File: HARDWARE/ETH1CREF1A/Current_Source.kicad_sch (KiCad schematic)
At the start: 25 parts, among them Q1102 BCP55, Q1103 BCP52, U1101 AD620, U1102 AD620

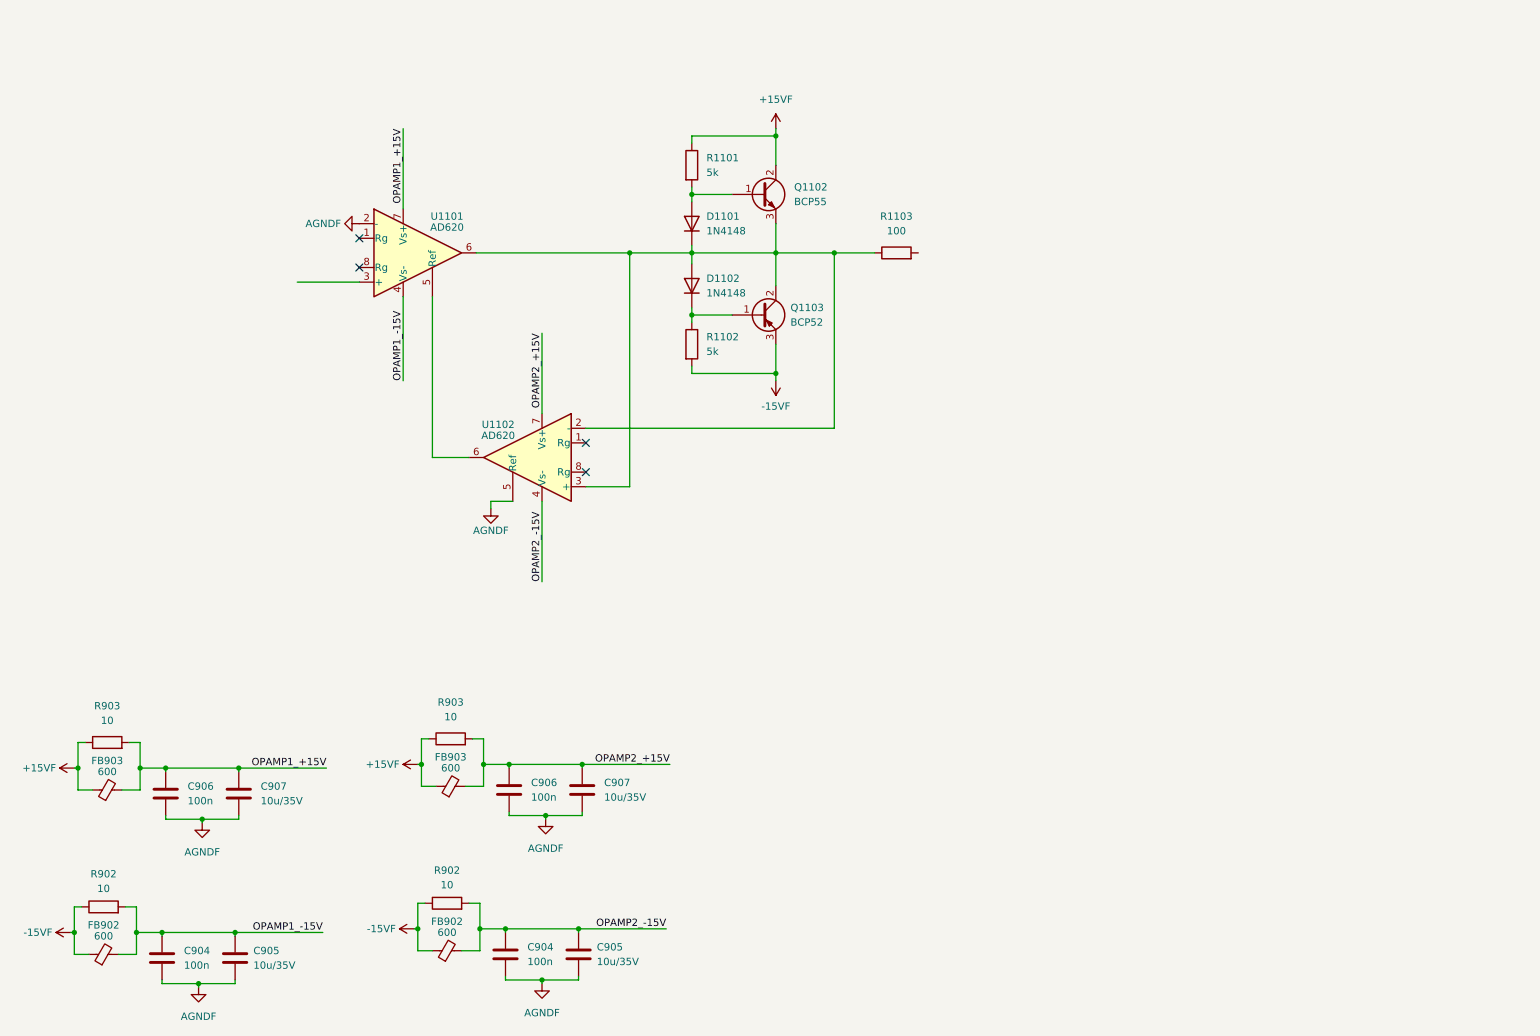
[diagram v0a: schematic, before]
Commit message: Hardware
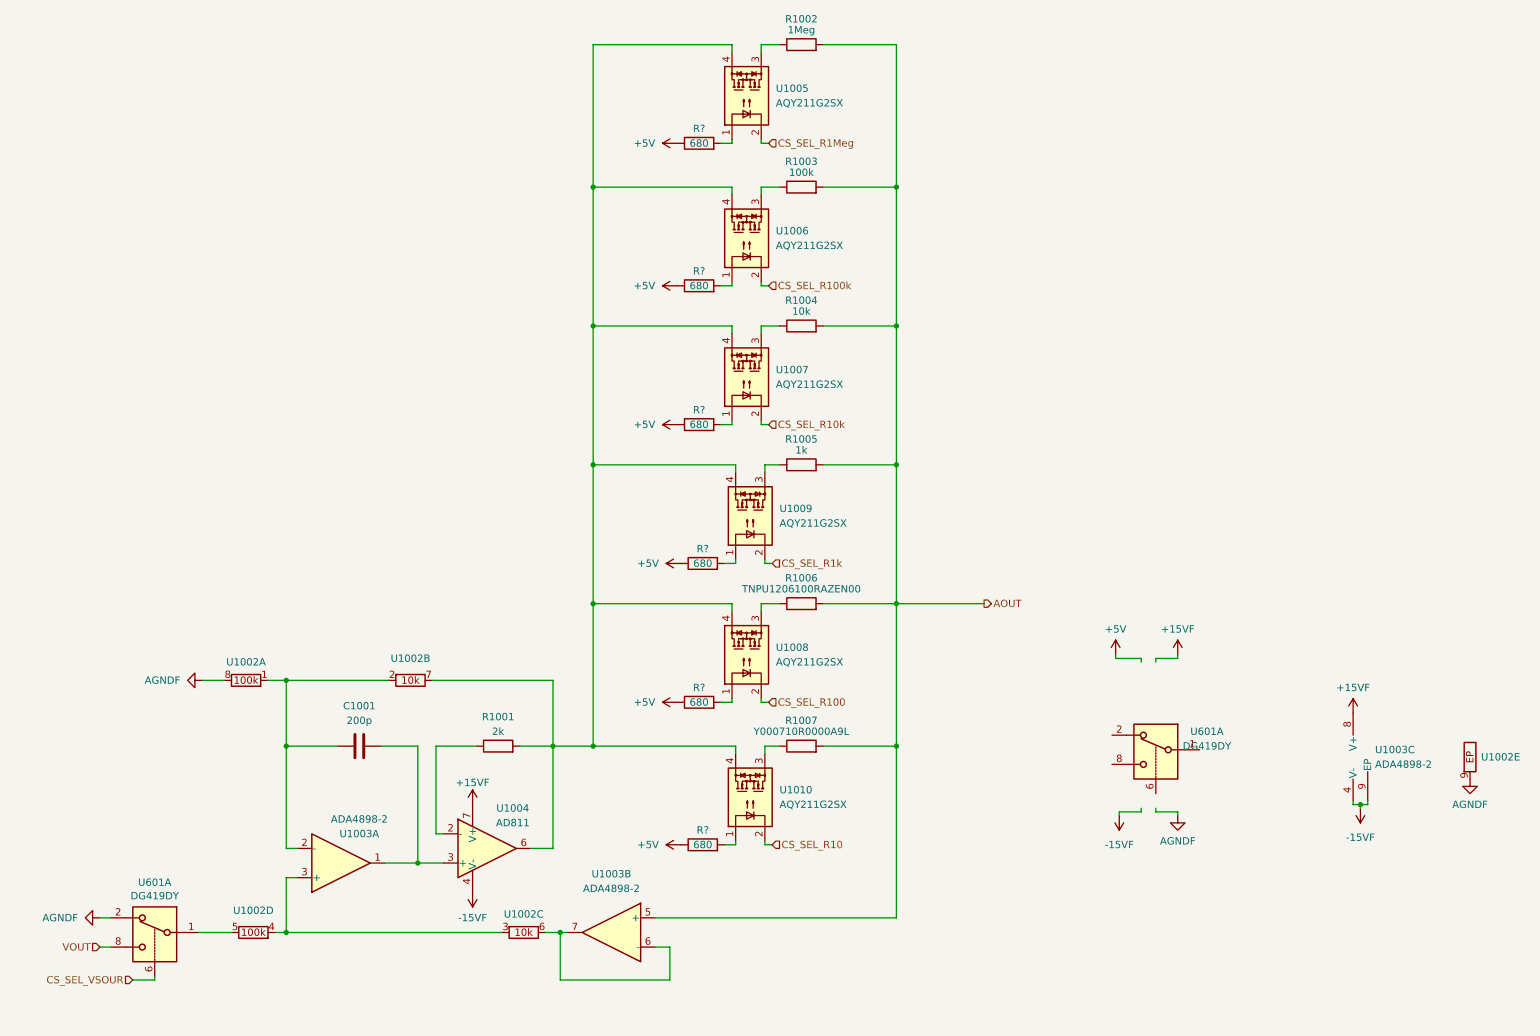
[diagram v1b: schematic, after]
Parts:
- removed C904 (x2), C906 (x2): 100n, symbol Device:C
- removed C905 (x2), C907 (x2): 10u/35V, symbol Device:C
- removed D1101, D1102: 1N4148, Diode_THT:D_DO-35_SOD27_P7.62mm_Horizontal, symbol Diode:1N4148
- removed FB902 (x2), FB903 (x2): 600, symbol Device:FerriteBead_Small
- removed Q1102: BCP55, Package_TO_SOT_SMD:SOT-223-3_TabPin2, symbol Transistor_BJT:BCP56
- removed Q1103: BCP52, Package_TO_SOT_SMD:SOT-223-3_TabPin2, symbol Transistor_BJT:BCP51
- removed R1101, R1102: 5k, symbol Device:R
- removed R1103: 100, symbol Device:R
- removed R902 (x2), R903 (x2): 10, symbol Device:R
- removed U1101, U1102: AD620, symbol Amplifier_Instrumentation:AD620
- added C1001: 200p, symbol Device:C
- added R1001: 2k, symbol Device:R
- added R1002: 1Meg, symbol Device:R
- added R1003: 100k, symbol Device:R
- added R1004: 10k, symbol Device:R
- added R1005: 1k, symbol Device:R
- added R1006: TNPU1206100RAZEN00, symbol Device:R
- added R1007: Y000710R0000A9L, symbol Device:R
- added R? (x6): 680, symbol Device:R
- added U1002: ~, symbol ETH1CREF1A:LT5400-3
- added U1003: ADA4898-2, Package_SO:SOIC-8-1EP_3.9x4.9mm_P1.27mm_EP2.41x3.81mm, symbol Amplifier_Operational:ADA4898-2
- added U1004: AD811, symbol ETH1CREF1A:AD811
- added U1005, U1006, U1007, U1008, U1009, U1010: AQY211G2SX, symbol ETH1CREF1A:AQY212GS
- added U601 (x2): DG419DY, Package_SO:SOIC-8_3.9x4.9mm_P1.27mm, symbol Analog_Switch:DG419xY
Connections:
- net +15VF: now also U1003.8 (V+), U1004.7 (V+)
- net -15VF: now also U1003.4 (V-), U1003.9 (EP), U1004.4 (V-)
- net AGNDF: now also U1002.8, U1002.9, U601.2
- new net: R?.2, U1008.1
- new net: R1006.1, U1008.3
- new net: R1001.2, U1002.7, U1004.6, U1005.4, U1006.4, U1007.4, U1008.4, U1009.4, U1010.4
- new net: U1002.5, U601.1
- new net: R1007.1, U1010.3
- new net: R1001.1, U1004.2 (-)
- new net: C1001.2, U1003.1, U1004.3 (+)
- new net: U1002.6, U1003.6 (-), U1003.7
- new net: C1001.1, U1002.1, U1002.2, U1003.2 (-)
- new net: U1002.3, U1002.4, U1003.3 (+)
- new net: R?.2, U1010.1
- new net: R?.2, U1009.1
- new net: R1005.1, U1009.3
- new net: R?.2, U1007.1
- new net: R1002.1, U1005.3
- new net: R1003.1, U1006.3
- new net: R?.2, U1005.1
- new net: R1004.1, U1007.3
- new net: R?.2, U1006.1
- new net +5V: R?.1, R?.1, R?.1, R?.1, R?.1, R?.1
- new net AOUT: R1002.2, R1003.2, R1004.2, R1005.2, R1006.2, R1007.2, U1003.5 (+)
- new net CS_SEL_R10: U1010.2
- new net CS_SEL_R100: U1008.2
- new net CS_SEL_R100k: U1006.2
- new net CS_SEL_R10k: U1007.2
- new net CS_SEL_R1Meg: U1005.2
- new net CS_SEL_R1k: U1009.2
- new net CS_SEL_VSOUR: U601.6
- new net VOUT: U601.8
- no-connect marks 4 -> 0
